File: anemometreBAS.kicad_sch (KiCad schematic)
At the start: 21 parts, among them U1 TP4056

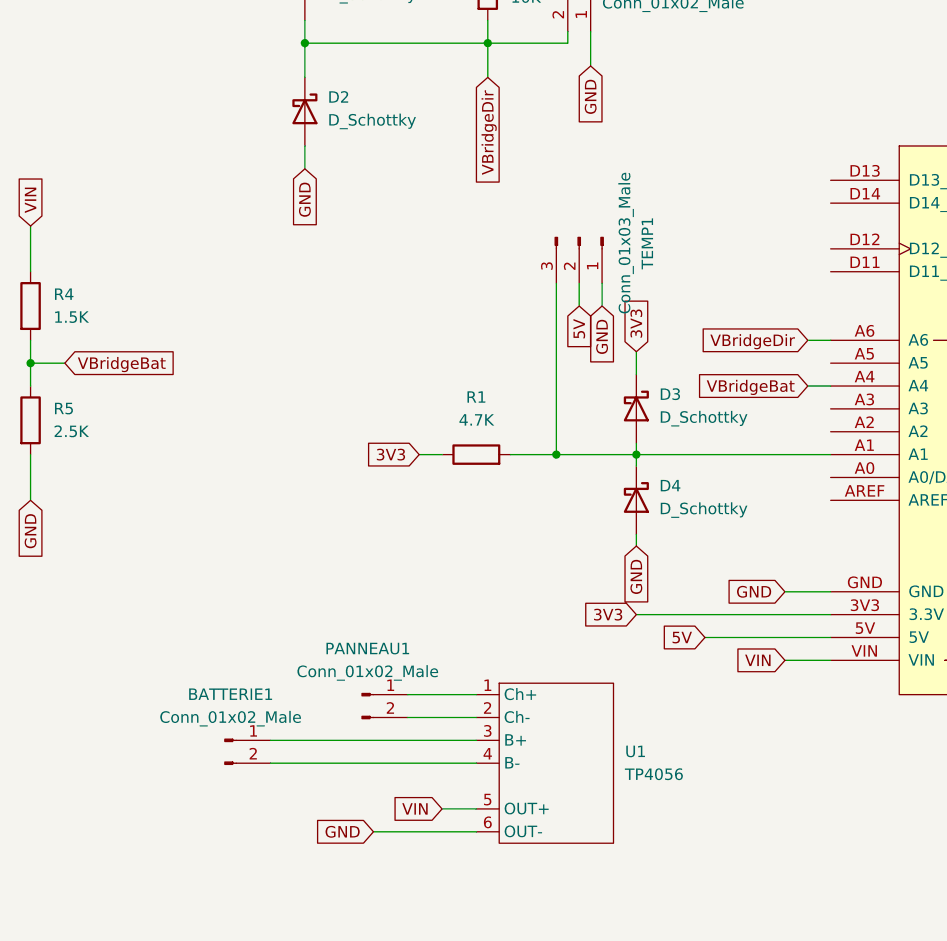
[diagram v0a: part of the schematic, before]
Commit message: Fix power issue
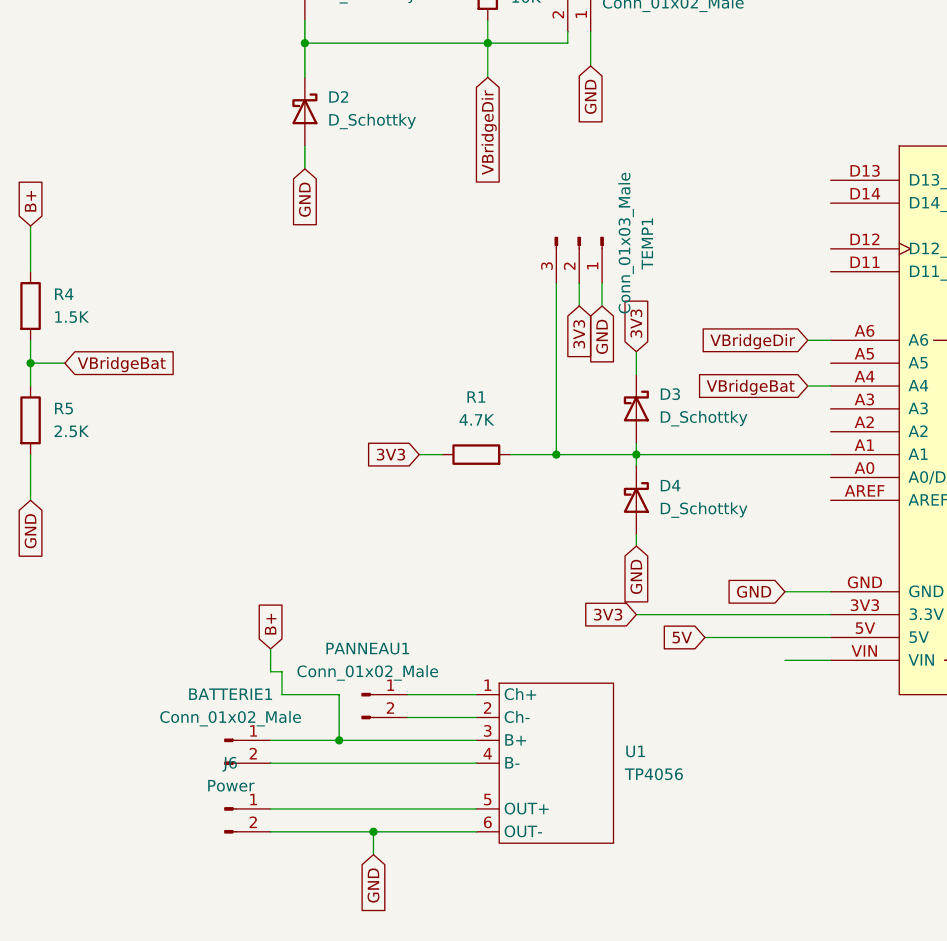
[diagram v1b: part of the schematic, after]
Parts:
- added J6: Power, symbol Connector:Conn_01x02_Male
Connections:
- net 3V3: now also TEMP1.2 (Pin_2)
- net 5V: no longer TEMP1.2 (Pin_2)
- net GND: now also J6.2 (Pin_2)
- net B+: now reaches BATTERIE1.1 (Pin_1), U1.3 (B+)
- net B+: now also R4.1
- removed net VIN: R4.1, U1.5 (OUT+), XA1.VIN
- new net: J6.1 (Pin_1), U1.5 (OUT+)
